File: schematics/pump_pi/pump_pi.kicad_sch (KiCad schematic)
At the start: 0 parts

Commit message: update schematics
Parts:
- added J1: Raspberry_Pi_4, symbol Connector:Raspberry_Pi_4
- added R1: 330, symbol Device:R
- added R2, R3, R4: 10k, symbol Device:R
- added RV1: R_Potentiometer, symbol Device:R_Potentiometer
- added SW1, SW2, SW3: SW_Push, symbol Switch:SW_Push
- added SW4: SW_Wuerth_450301014042, Button_Switch_THT:SW_Slide-03_Wuerth-WS-SLTV_10x2.5x6.4_P2.54mm, symbol Switch:SW_Wuerth_450301014042
- added U1: MCP3008, symbol Analog_ADC:MCP3008
- added U2: TLP3542, Package_DIP:DIP-5-6_W7.62mm, symbol Relay_SolidState:TLP3542
- added U3: Vacuum sensor, symbol shm_symbols:Vacuum_sensor
- added U4: Voltage meter, symbol shm_symbols:Voltage_meter
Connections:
- new net: SW4.1 (B), U1.1 (CH0), U4. (Black)
- new net: RV1.2, SW4.2 (C)
- new net: SW4.3 (A), U3. (Black)
- new net: R1.1, U2.1
- new net: J1.14 (GND), J1.20 (GND), J1.25 (GND), J1.30 (GND), J1.34 (GND), J1.39 (GND), J1.6 (GND), J1.9 (GND), R2.1, R3.1, R4.1, RV1.1, U1.14 (AGND), U1.9 (DGND), U2.2, U3. (Black), U4. (Black)
- new net: J1.1 (3V3), J1.17 (3V3)
- new net: J1.15 (GPIO22/SDIO_CLK), R1.2
- new net: J1.19 (MOSI_SPI0/GPIO10), U1.11 (Din)
- new net: J1.2 (5V), J1.4 (5V), RV1.3, SW1.2, SW2.2, SW3.2, U1.15 (Vref), U1.16 (Vdd), U3. (Black), U4. (Black)
- new net: J1.21 (MISO_SPI0/GPIO09), U1.12 (Dout)
- new net: J1.23 (SCLK_SPI0/GPIO11), U1.13 (CLK)
- new net: J1.29 (GPCLK1/GPIO05), U1.10 (~{CS}/SHDN)
- new net: R4.2, SW3.1, U1.4 (CH3)
- new net: R2.2, SW1.1, U1.2 (CH1)
- new net: R3.2, SW2.1, U1.3 (CH2)
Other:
- note added: "Auto pump on"
- note added: "Manual pump on"
- note added: "Tank empty pump off"

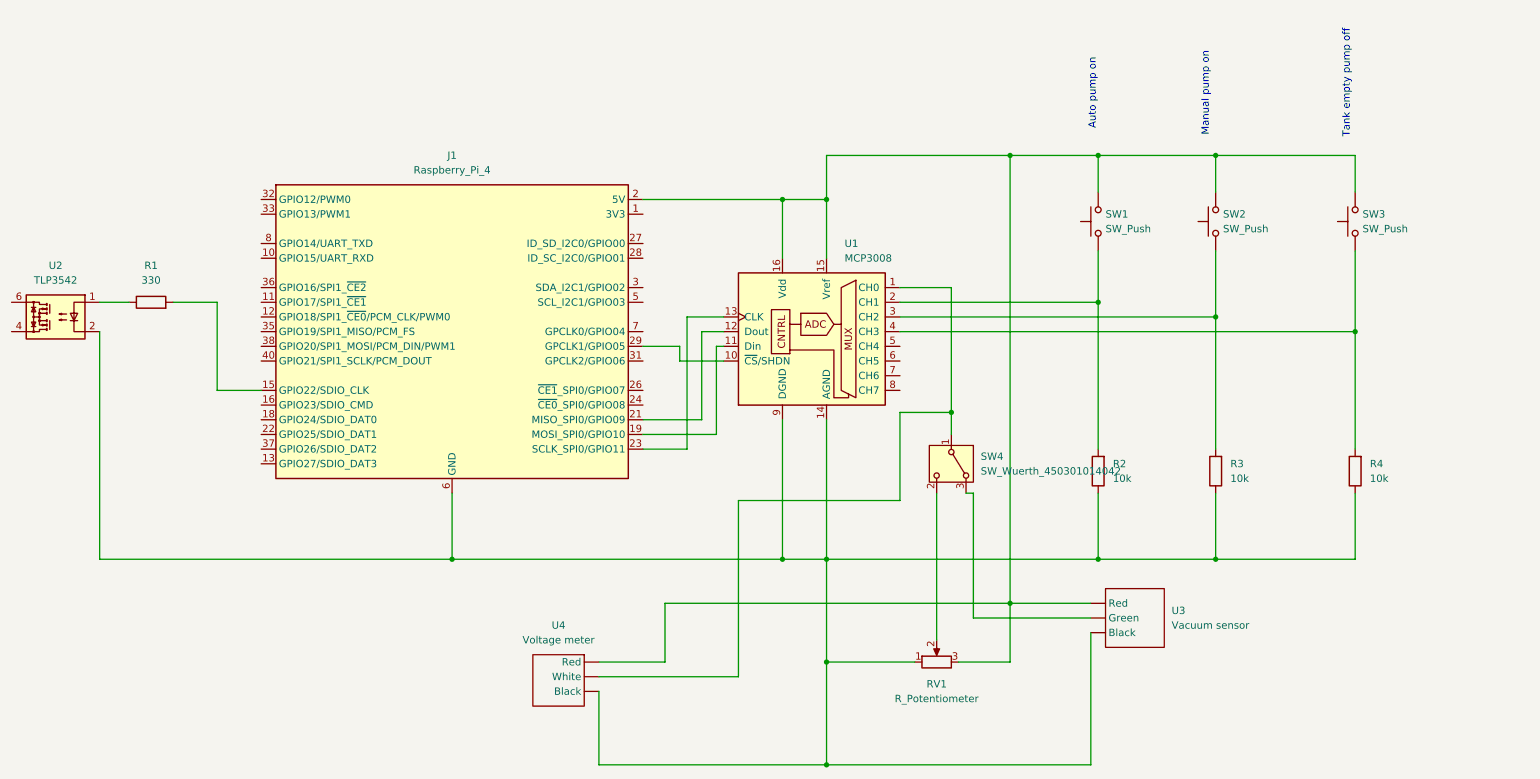
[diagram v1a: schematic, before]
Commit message: update schematics
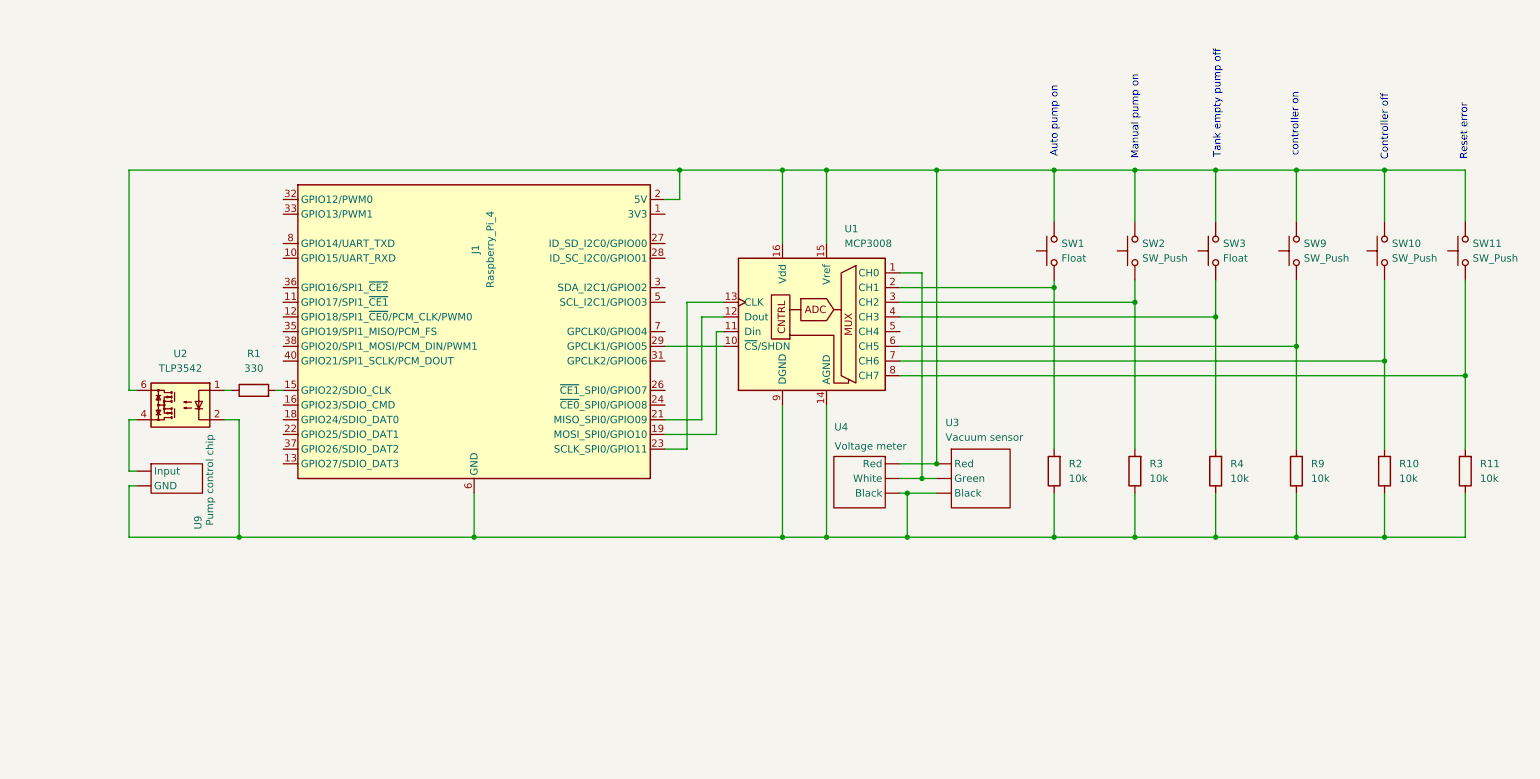
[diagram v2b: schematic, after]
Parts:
- removed RV1: R_Potentiometer, symbol Device:R_Potentiometer
- removed SW4: SW_Wuerth_450301014042, Button_Switch_THT:SW_Slide-03_Wuerth-WS-SLTV_10x2.5x6.4_P2.54mm, symbol Switch:SW_Wuerth_450301014042
- added R10, R11, R9: 10k, symbol Device:R
- added SW10, SW11, SW9: SW_Push, symbol Switch:SW_Push
- added U9: Pump control chip, symbol shm_symbols:Pump_control_chip
- SW1, SW3: value SW_Push -> Float
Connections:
- net at U1.1 (CH0), U4. (Black): now also U3. (Black)
- net at J1.14 (GND), J1.20 (GND), J1.25 (GND)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: now also R10.1, R11.1, R9.1, U9. (GND)
- net at U2.4: now also U9. (GND)
- net at U2.6: now also J1.2 (5V), J1.4 (5V), SW1.2, SW2.2, SW3.2, U1.15 (Vref), U1.16 (Vdd), U3. (Black), U4. (Black), SW10.2, SW11.2, SW9.2
- net at U1.6 (CH5): now also R9.2, SW9.1
- net at U1.7 (CH6): now also R10.2, SW10.1
- net at U1.8 (CH7): now also R11.2, SW11.1
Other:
- note added: "Controller off"
- note added: "Reset error"
- note added: "controller on"
- moved on the sheet: J1, R1, R2, R3, R4, SW1, SW2, SW3, U1, U2, U3, U4

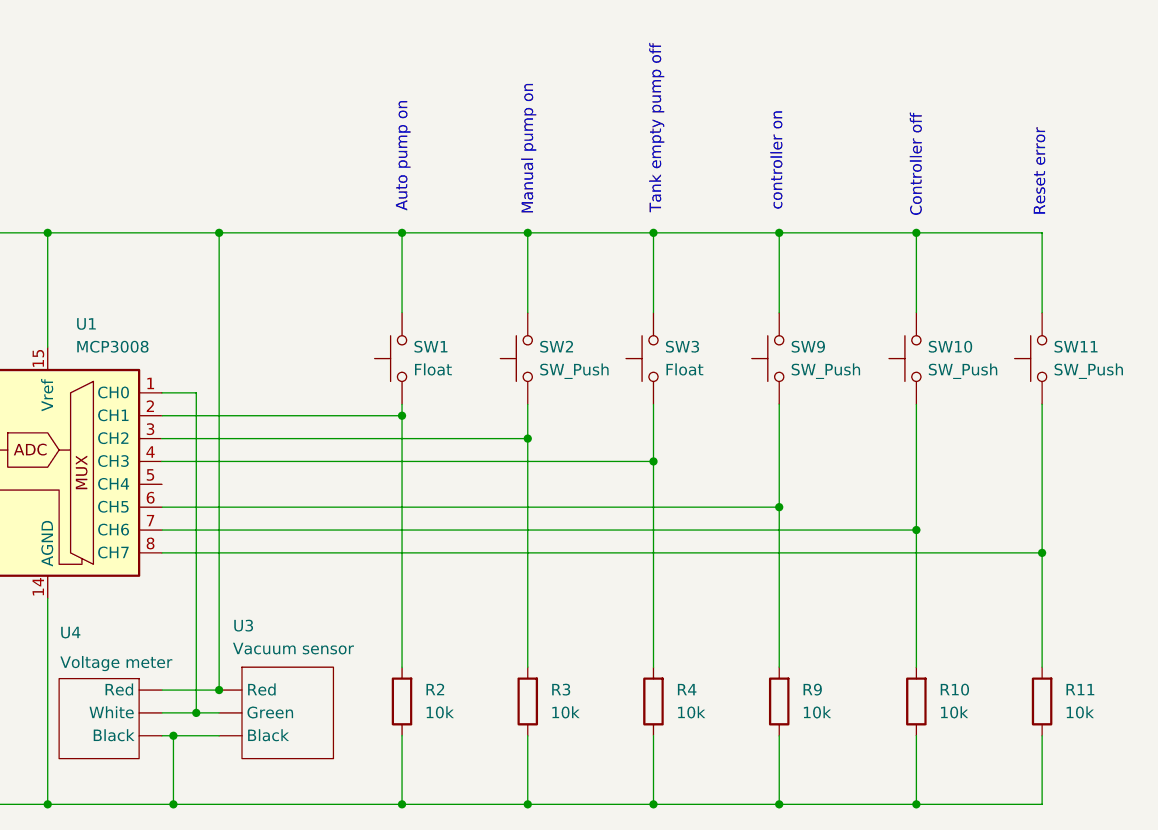
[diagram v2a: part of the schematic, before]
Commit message: update schematics
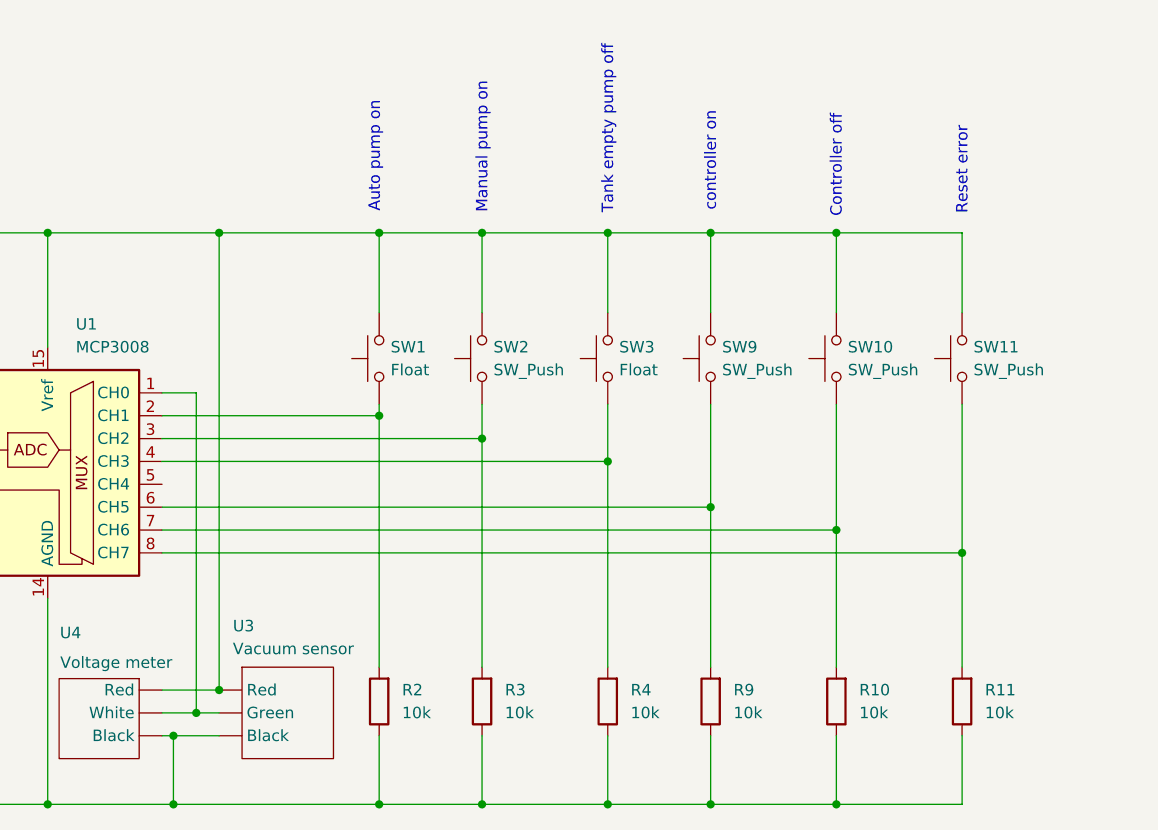
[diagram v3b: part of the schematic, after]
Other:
- moved on the sheet: R10, R11, R2, R3, R4, R9, SW1, SW10, SW11, SW2, SW3, SW9
